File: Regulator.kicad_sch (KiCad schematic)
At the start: 26 parts, among them J1 Conn_01x04_Pin, Q1 D965L, Q2 C1815L, Q3 C1815L, Q4 TIP107, Q5 A1015L

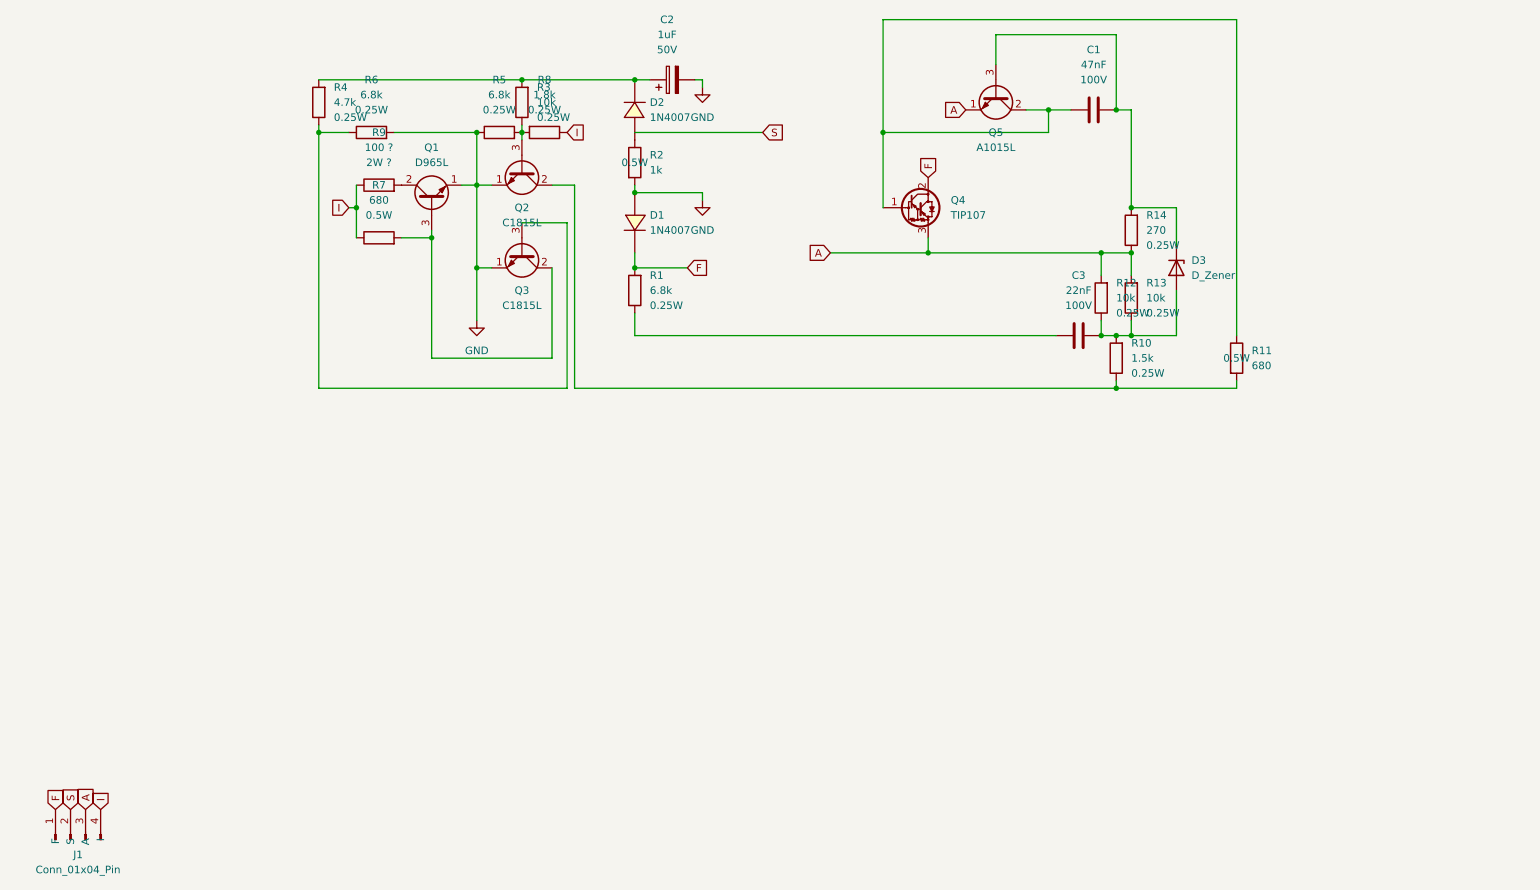
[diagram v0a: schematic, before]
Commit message: Routing and layout done
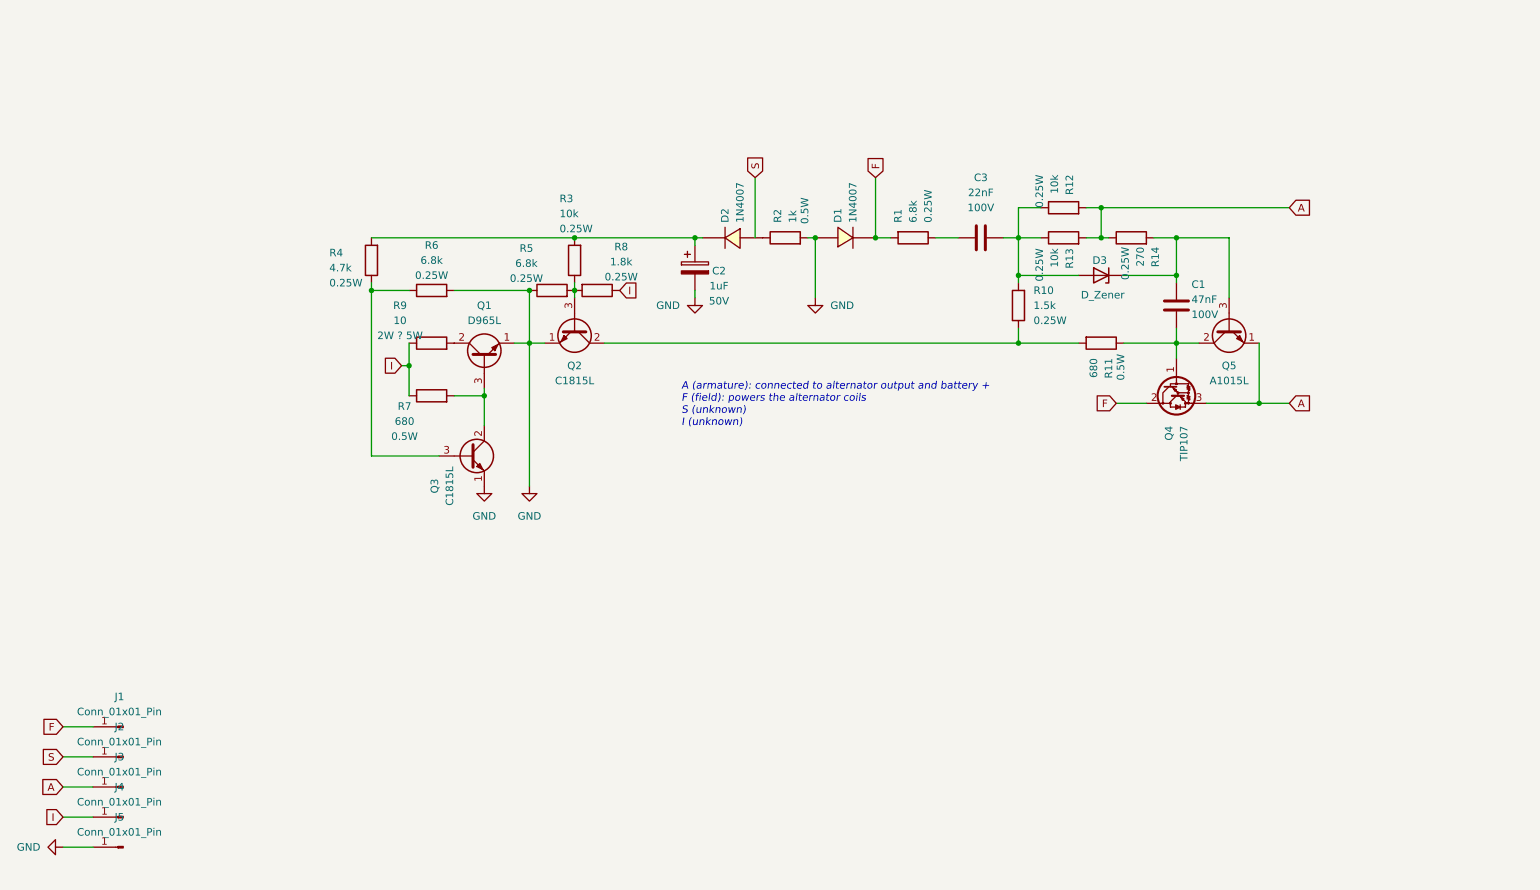
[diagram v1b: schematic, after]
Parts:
- removed J1: Conn_01x04_Pin, Connector_PinHeader_2.54mm:PinHeader_1x04_P2.54mm_Vertical, symbol Connector:Conn_01x04_Pin
- added J1, J2, J3, J4, J5: Conn_01x01_Pin, Connector_Wire:SolderWire-6sqmm_1x01_D3.5mm_OD7mm, symbol Connector:Conn_01x01_Pin
- R1, R10, R12, R13, R14, R3, R4, R5, R6, R8: footprint Resistor_THT:R_Axial_DIN0204_L3.6mm_D1.6mm_P5.08mm_Horizontal -> Resistor_THT:R_Axial_DIN0207_L6.3mm_D2.5mm_P10.16mm_Horizontal
- R11, R2, R7: footprint Resistor_THT:R_Axial_DIN0204_L3.6mm_D1.6mm_P5.08mm_Horizontal -> Resistor_THT:R_Axial_DIN0309_L9.0mm_D3.2mm_P15.24mm_Horizontal
- R9: value 100 ? -> 10; footprint Resistor_THT:R_Axial_DIN0204_L3.6mm_D1.6mm_P5.08mm_Horizontal -> Resistor_THT:R_Axial_DIN0516_L15.5mm_D5.0mm_P20.32mm_Horizontal; Power 2W ? -> 2W ? 5W
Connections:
- net A: now also J3.1 (Pin_1)
- net F: now also J1.1 (Pin_1)
- net GND: now also J5.1 (Pin_1)
- net I: now also J4.1 (Pin_1)
- net S: now also J2.1 (Pin_1)
- net at Q4.1 (B), Q5.2 (C), R11.1: now also C1.2; no longer C1.1
- net at D3.1 (K), Q5.3 (B), R14.2: now also C1.1; no longer C1.2
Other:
- note added: "A (armature): connected to alternator output and battery + F (field): powers the alternator coils S (unknown) I (unknown)"
- moved on the sheet: C1, C2, C3, D1, D2, D3, Q1, Q2, Q3, Q4, Q5, R1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

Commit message: Started simulation work for circuit
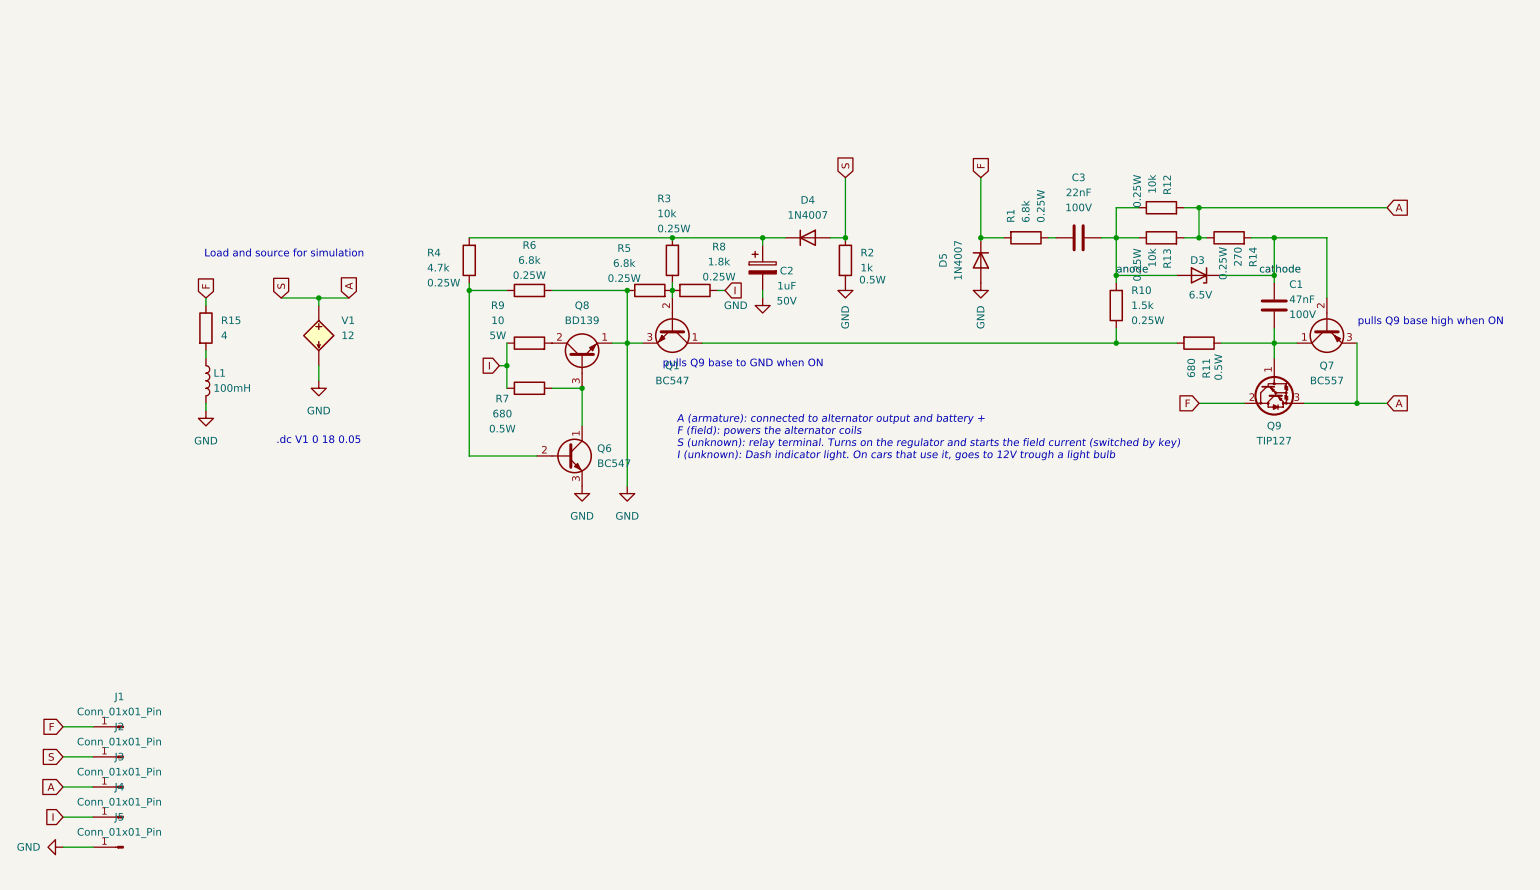
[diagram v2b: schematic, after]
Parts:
- removed D1, D2: 1N4007, Diode_THT:D_A-405_P7.62mm_Horizontal, symbol mustang_regulator:1N4007
- removed Q1: D965L, Package_TO_SOT_THT:TO-92_Inline, symbol Transistor_BJT:Q_NPN_ECB
- removed Q2, Q3: C1815L, Package_TO_SOT_THT:TO-92_Inline, symbol Transistor_BJT:Q_NPN_ECB
- removed Q4: TIP107, Package_TO_SOT_THT:TO-220-3_Vertical, symbol Transistor_BJT:TIP127
- removed Q5: A1015L, Package_TO_SOT_THT:TO-92_Inline, symbol Transistor_BJT:Q_NPN_ECB
- added D4, D5: 1N4007, Diode_THT:D_DO-41_SOD81_P10.16mm_Horizontal, symbol Diode:1N4007
- added L1: 100mH, symbol Device:L
- added Q1, Q6: BC547, Package_TO_SOT_THT:TO-92_Inline, symbol Transistor_BJT:BC547
- added Q7: BC557, Package_TO_SOT_THT:TO-92_Inline, symbol Transistor_BJT:BC557
- added Q8: BD139, Package_TO_SOT_THT:TO-126-3_Vertical, symbol Transistor_BJT:BD139
- added Q9: TIP127, Package_TO_SOT_THT:TO-220-3_Vertical, symbol Transistor_BJT:TIP127
- added R15: 4, symbol Device:R
- added V1: 12, symbol Simulation_SPICE:BSOURCE
- D3: value D_Zener -> 6.5V
- R9: Power 2W ? 5W -> 5W
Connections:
- net S is gone; now on net A: J2.1 (Pin_1)
- net A: now also R2.1, D4.2 (A), Q7.3 (E), Q9.3 (E), V1.1 (N+)
- net F: now also D5.1 (K), Q9.2 (C), R15.1
- net GND: now also D5.2 (A), L1.2, Q1.3 (E), Q6.3 (E), Q8.1 (E), V1.2 (N-)
- net at R9.2: now also Q8.2 (C)
- net at R10.1, R11.2: now also Q1.1 (C)
- net at R3.1, R5.2, R8.2: now also Q1.2 (B)
- net cathode: now reaches C1.1, D3.1 (K), R14.2
- net cathode: now also Q7.2 (B)
- net at C1.2, R11.1: now also Q7.1 (C), Q9.1 (B)
- net anode: now reaches C3.2, D3.2 (A), R10.2, R12.1, R13.1
- net at C2.1, R3.2, R4.2: now also D4.1 (K)
- net at R4.1, R6.1: now also Q6.2 (B)
- net at R7.2: now also Q6.1 (C), Q8.3 (B)
- new net: L1.1, R15.2
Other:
- note added: ".dc V1 0 18 0.05"
- note added: "A (armature): connected to alternator output and battery + F (field): powers the alternator coils S (unknown): relay terminal. Turns on the regulator and starts the field current (switched by key) I (unknown): Dash indicator light. On cars that use it, goes to 12V trough a light bulb"
- note added: "Load and source for simulation"
- note added: "pulls Q9 base high when ON"
- note added: "pulls Q9 base to GND when ON"
- note removed: "A (armature): connected to alternator output and battery + F (field): powers the alternator coils S (unknown) I (unknown)"
- moved on the sheet: C1, C2, C3, D3, R1, R10, R11, R12, R13, R14, R2, R3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
